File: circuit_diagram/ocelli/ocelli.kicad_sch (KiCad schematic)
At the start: 114 parts, among them J1 Conn_01x06, J2 Conn_01x06, J3 Conn_01x06, J4 Conn_01x06, J5 Conn_01x08, J6 Conn_01x02, J7 Conn_01x02, Q1 BSS138, Q10 BSS138, Q2 ST-1KL3A, Q3 TJ8S06M3L, Q4 ST-1KL3A, Q5 BSS138, Q6 ST-1KL3A, Q7 BSS138, Q8 ST-1KL3A, Q9 BSS138, SW1 SW_SPDT, SW2 TVAF06-A020B-R, SW3 TVAF06-A020B-R, SW4 TVAF06-A020B-R, SW5 TVAF06-A020B-R, SW6 TVAF06-A020B-R, U1 NJM2845DL1-33, U2 AS5055A, U3 AS5055A, U4 ICM-20649, U5 STM32F405RGTx, U6 DRV8835

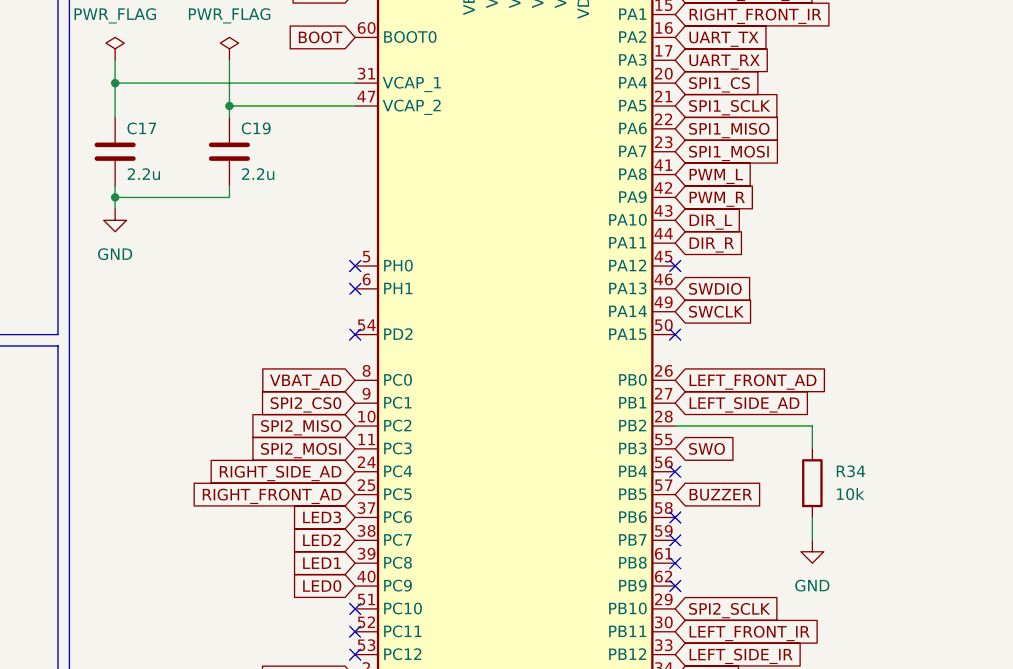
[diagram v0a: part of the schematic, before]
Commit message: 一通りパターンを繋いだ
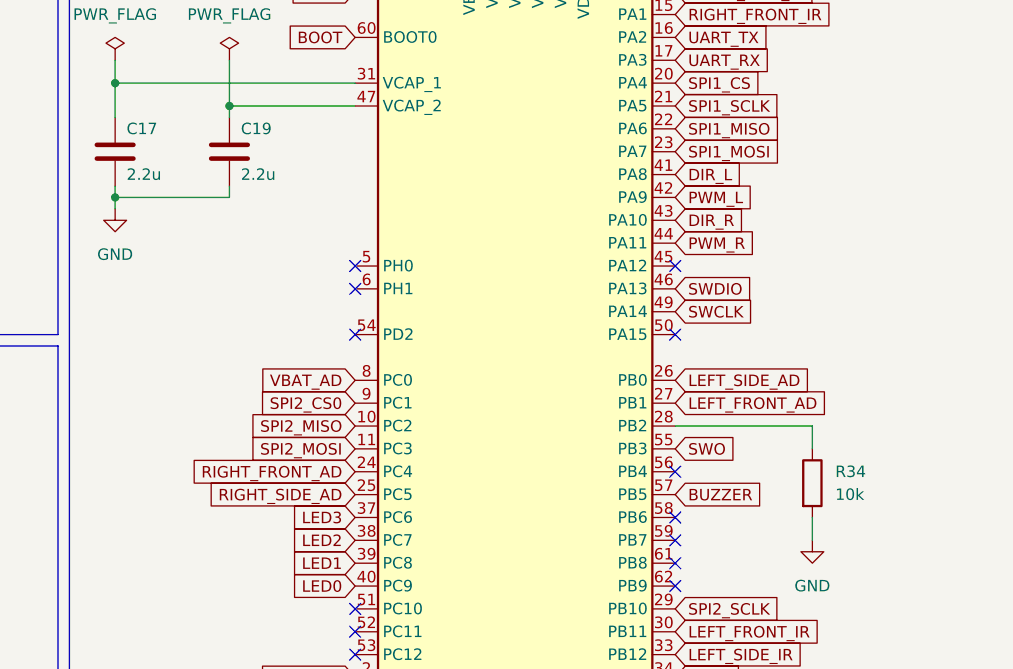
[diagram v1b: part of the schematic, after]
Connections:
- net DIR_L: now also U5.41 (PA8); no longer U5.43 (PA10)
- net DIR_R: now also U5.43 (PA10); no longer U5.44 (PA11)
- net LEFT_FRONT_AD: now also U5.27 (PB1); no longer U5.26 (PB0)
- net LEFT_SIDE_AD: now also U5.26 (PB0); no longer U5.27 (PB1)
- net PWM_L: now also U5.42 (PA9); no longer U5.41 (PA8)
- net PWM_R: now also U5.44 (PA11); no longer U5.42 (PA9)
- net RIGHT_FRONT_AD: now also U5.24 (PC4); no longer U5.25 (PC5)
- net RIGHT_SIDE_AD: now also U5.25 (PC5); no longer U5.24 (PC4)
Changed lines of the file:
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@@
     )
   )
-  (global_label "RIGHT_SIDE_AD" (shape input) (at 233.68 185.42 180) (fields_autoplaced)
-    (effects (font (size 1.27 1.27)) (justify right))
-    (property "Intersheet References" "${INTERSHEET_REFS}" (id 0) (at 217.2969 185.4994 0)
+  (global_label "RIGHT_SIDE_AD" (shape input) (at 233.68 187.96 180) (fields_autoplaced)
+    (effects (font (size 1.27 1.27)) (justify right))
+    (property "Intersheet References" "${INTERSHEET_REFS}" (id 0) (at 217.2969 188.0394 0)
       (effects (font (size 1.27 1.27)) (justify right) hide)
     )
@@
     )
   )
-  (global_label "LEFT_FRONT_AD" (shape input) (at 269.24 175.26 0) (fields_autoplaced)
-    (effects (font (size 1.27 1.27)) (justify left))
-    (property "Intersheet References" "${INTERSHEET_REFS}" (id 0) (at 286.1674 175.1806 0)
-      (effects (font (size 1.27 1.27)) (justify left) hide)
-    )
-  )
-  (global_label "RIGHT_FRONT_AD" (shape input) (at 233.68 187.96 180) (fields_autoplaced)
-    (effects (font (size 1.27 1.27)) (justify right))
-    (property "Intersheet References" "${INTERSHEET_REFS}" (id 0) (at 215.5431 188.0394 0)
+  (global_label "LEFT_FRONT_AD" (shape input) (at 269.24 177.8 0) (fields_autoplaced)
+    (effects (font (size 1.27 1.27)) (justify left))
+    (property "Intersheet References" "${INTERSHEET_REFS}" (id 0) (at 286.1674 177.7206 0)
+      (effects (font (size 1.27 1.27)) (justify left) hide)
+    )
+  )
+  (global_label "RIGHT_FRONT_AD" (shape input) (at 233.68 185.42 180) (fields_autoplaced)
+    (effects (font (size 1.27 1.27)) (justify right))
+    (property "Intersheet References" "${INTERSHEET_REFS}" (id 0) (at 215.5431 185.4994 0)
       (effects (font (size 1.27 1.27)) (justify right) hide)
     )
@@
     )
   )
-  (global_label "DIR_L" (shape input) (at 269.24 157.48 0) (fields_autoplaced)
-    (effects (font (size 1.27 1.27)) (justify left))
-    (property "Intersheet References" "${INTERSHEET_REFS}" (id 0) (at 276.7936 157.4006 0)
+  (global_label "DIR_L" (shape input) (at 269.24 152.4 0) (fields_autoplaced)
+    (effects (font (size 1.27 1.27)) (justify left))
+    (property "Intersheet References" "${INTERSHEET_REFS}" (id 0) (at 276.7936 152.3206 0)
       (effects (font (size 1.27 1.27)) (justify left) hide)
     )
@@
     )
   )
-  (global_label "LEFT_SIDE_AD" (shape input) (at 269.24 177.8 0) (fields_autoplaced)
-    (effects (font (size 1.27 1.27)) (justify left))
-    (property "Intersheet References" "${INTERSHEET_REFS}" (id 0) (at 284.4136 177.7206 0)
+  (global_label "LEFT_SIDE_AD" (shape input) (at 269.24 175.26 0) (fields_autoplaced)
+    (effects (font (size 1.27 1.27)) (justify left))
+    (property "Intersheet References" "${INTERSHEET_REFS}" (id 0) (at 284.4136 175.1806 0)
       (effects (font (size 1.27 1.27)) (justify left) hide)
     )
@@
     )
   )
-  (global_label "PWM_R" (shape input) (at 269.24 154.94 0) (fields_autoplaced)
-    (effects (font (size 1.27 1.27)) (justify left))
-    (property "Intersheet References" "${INTERSHEET_REFS}" (id 0) (at 278.0636 154.8606 0)
+  (global_label "PWM_R" (shape input) (at 269.24 160.02 0) (fields_autoplaced)
+    (effects (font (size 1.27 1.27)) (justify left))
+    (property "Intersheet References" "${INTERSHEET_REFS}" (id 0) (at 278.0636 159.9406 0)
       (effects (font (size 1.27 1.27)) (justify left) hide)
     )
@@
     )
   )
-  (global_label "PWM_L" (shape input) (at 269.24 152.4 0) (fields_autoplaced)
-    (effects (font (size 1.27 1.27)) (justify left))
-    (property "Intersheet References" "${INTERSHEET_REFS}" (id 0) (at 277.8217 152.3206 0)
+  (global_label "PWM_L" (shape input) (at 269.24 154.94 0) (fields_autoplaced)
+    (effects (font (size 1.27 1.27)) (justify left))
+    (property "Intersheet References" "${INTERSHEET_REFS}" (id 0) (at 277.8217 154.8606 0)
       (effects (font (size 1.27 1.27)) (justify left) hide)
     )
@@
     )
   )
-  (global_label "DIR_R" (shape input) (at 269.24 160.02 0) (fields_autoplaced)
-    (effects (font (size 1.27 1.27)) (justify left))
-    (property "Intersheet References" "${INTERSHEET_REFS}" (id 0) (at 277.0355 159.9406 0)
-      (effects (font (size 1.27 1.27)) (justify left) hide)
-    )
+  (global_label "DIR_R" (shape input) (at 269.24 157.48 0) (fields_autoplaced)
+    (effects (font (size 1.27 1.27)) (justify left))
+    (property "Intersheet References" "${INTERSHEET_REFS}" (id 0) (at 277.0355 157.4006 0)
+      (effects (font (size 1.27 1.27)) (justify left) hide)
+    )
